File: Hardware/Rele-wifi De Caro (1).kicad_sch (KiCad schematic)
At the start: 38 parts, among them IC1 MC7805CD2TG, J1 Screw_Terminal_01x03, J2 Screw_Terminal_01x03, J3 Screw_Terminal_01x03, J4 Screw_Terminal_01x03, J5 Screw_Terminal_01x02, K1 PR13-5V-450-1C, K2 PR13-5V-450-1C, K3 PR13-5V-450-1C, K4 PR13-5V-450-1C, Q1 PC817-B, Q2 PC817-B, Q3 BC547, Q4 BC547, Q5 PC817-B, Q6 BC547, Q7 PC817-B, Q8 BC547, SW1 SW_DPST_x2, U2 ESP32-CAM

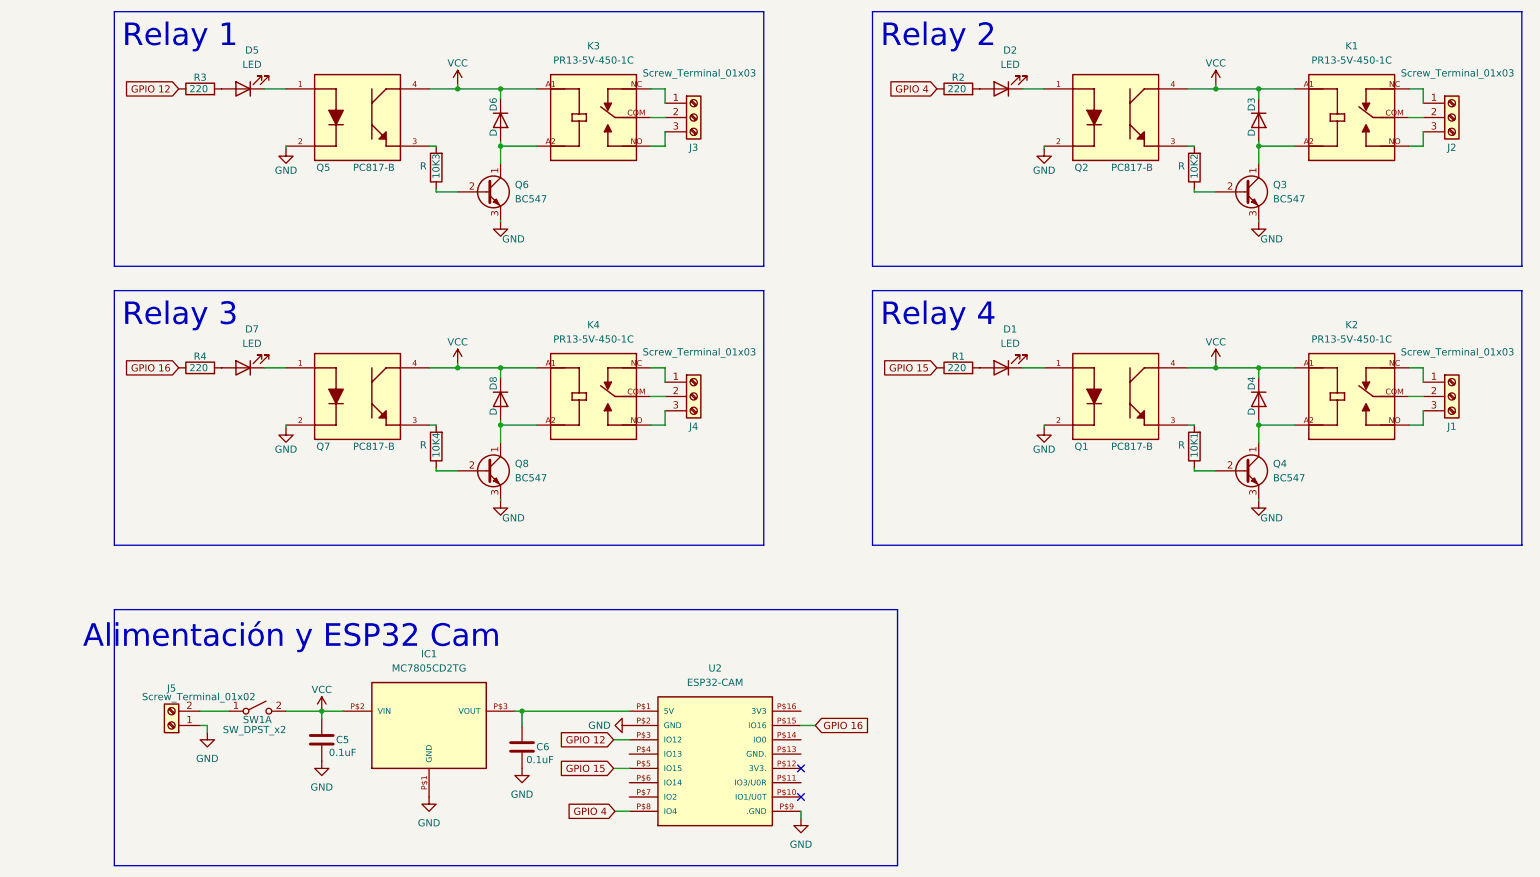
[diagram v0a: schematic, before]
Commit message: PCB terminado 2.0
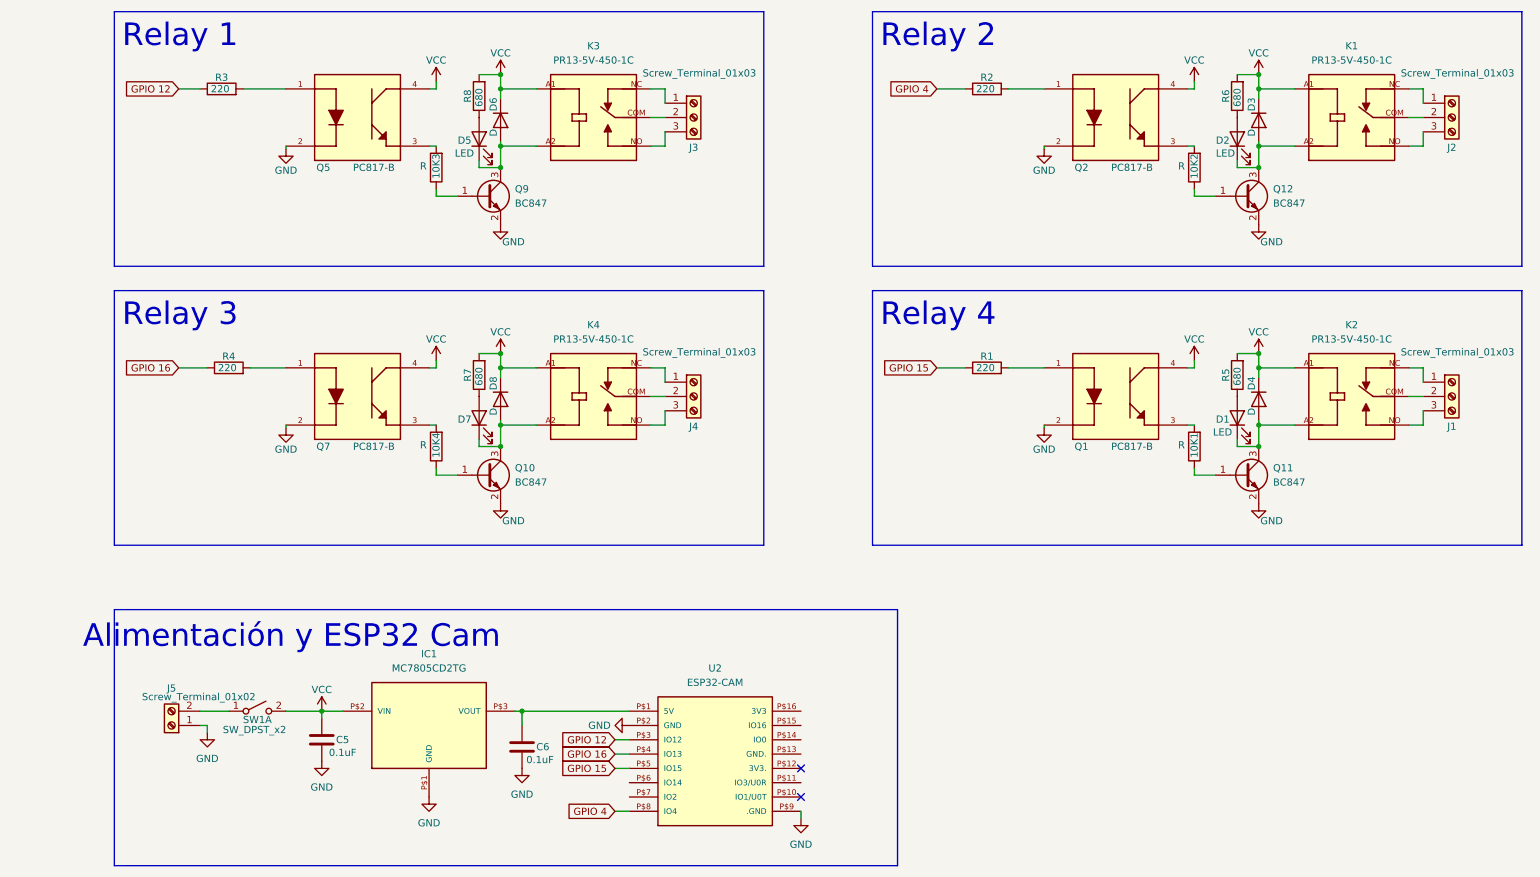
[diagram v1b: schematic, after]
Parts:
- removed Q3, Q4, Q6, Q8: BC547, bc547 smd:SOT95P230X110-3N, symbol EESTN5:BC547
- added Q10, Q11, Q12, Q9: BC847, Package_TO_SOT_SMD:SOT-23, symbol Transistor_BJT:BC847
- added R5, R6, R7, R8: 680, Resistor_SMD:R_0805_2012Metric_Pad1.20x1.40mm_HandSolder, symbol Device:R
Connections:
- net GND: now also Q10.2 (E), Q11.2 (E), Q12.2 (E), Q9.2 (E)
- net GPIO 16: now also U2.P$4 (IO13); no longer U2.P$15 (IO16)
- net VCC: now also R5.2, R6.2, R7.2, R8.2
- net at D3.2 (A), K1.A2: now also D2.1 (K), Q12.3 (C)
- net at Q1.1: now also R1.2; no longer D1.1 (K)
- net at 10K1.1: now also Q11.1 (B)
- net at R4.2: now also Q7.1; no longer D7.2 (A)
- net at 10K2.1: now also Q12.1 (B)
- net at D7.1 (K): now also D8.2 (A), K4.A2, Q10.3 (C); no longer Q7.1
- net at D5.2 (A): now also R8.1; no longer R3.2
- net at Q5.1: now also R3.2; no longer D5.1 (K)
- net at D6.2 (A), K3.A2: now also D5.1 (K), Q9.3 (C)
- net at D4.2 (A), K2.A2: now also D1.1 (K), Q11.3 (C)
- net at 10K4.1: now also Q10.1 (B)
- net at R2.2: now also Q2.1; no longer D2.2 (A)
- net at 10K3.1: now also Q9.1 (B)
- net at D1.2 (A): now also R5.1; no longer R1.2
- new net: D7.2 (A), R7.1
- new net: D2.2 (A), R6.1
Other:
- moved on the sheet: D1, D2, D5, D7, R1, R3, R4
